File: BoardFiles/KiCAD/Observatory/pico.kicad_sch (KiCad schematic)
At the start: 2 parts, among them J31 Jumper, U5 Pico

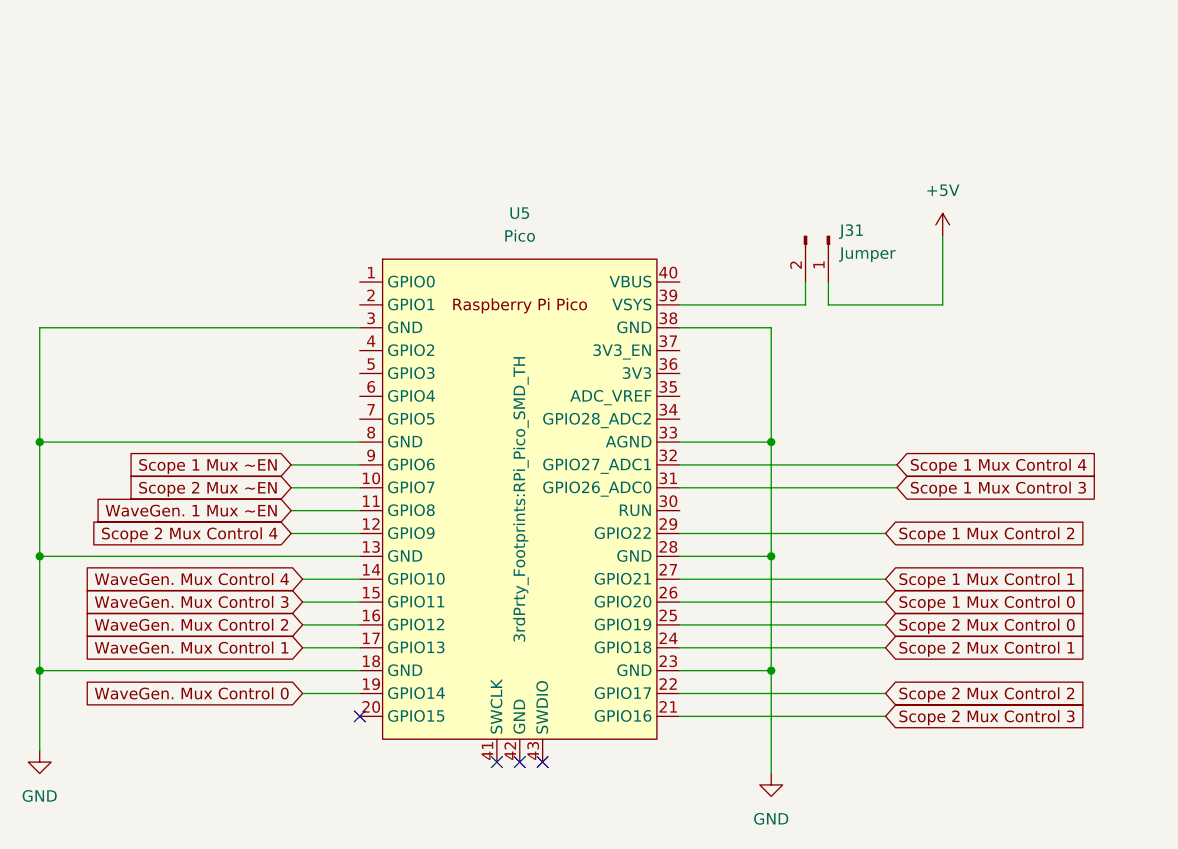
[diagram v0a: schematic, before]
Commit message: REV3 begin
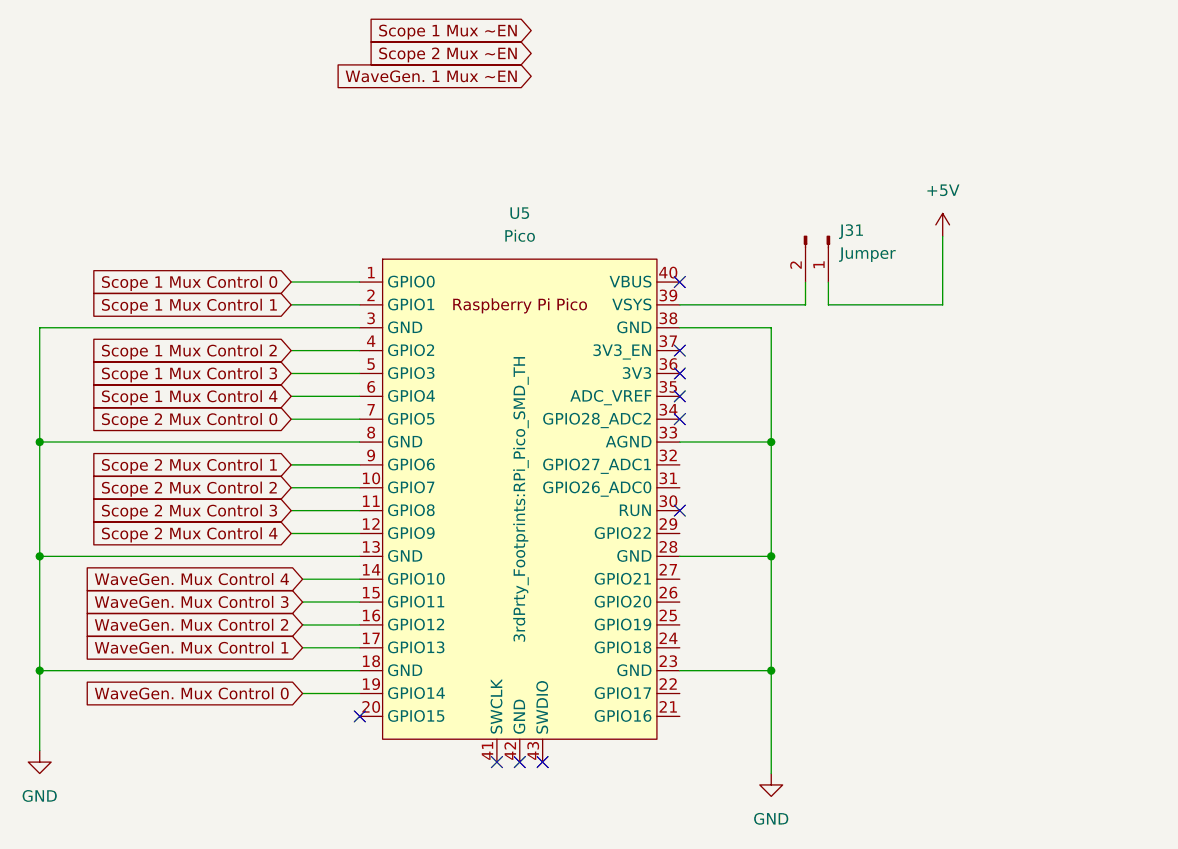
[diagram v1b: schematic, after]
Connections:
- net Scope 1 Mux Control 0: now also U5.1 (GPIO0); no longer U5.26 (GPIO20)
- net Scope 1 Mux Control 1: now also U5.2 (GPIO1); no longer U5.27 (GPIO21)
- net Scope 1 Mux Control 2: now also U5.4 (GPIO2); no longer U5.29 (GPIO22)
- net Scope 1 Mux Control 3: now also U5.5 (GPIO3); no longer U5.31 (GPIO26_ADC0)
- net Scope 1 Mux Control 4: now also U5.6 (GPIO4); no longer U5.32 (GPIO27_ADC1)
- net Scope 1 Mux ~EN: no longer U5.9 (GPIO6)
- net Scope 2 Mux Control 0: now also U5.7 (GPIO5); no longer U5.25 (GPIO19)
- net Scope 2 Mux Control 1: now also U5.9 (GPIO6); no longer U5.24 (GPIO18)
- net Scope 2 Mux Control 2: now also U5.10 (GPIO7); no longer U5.22 (GPIO17)
- net Scope 2 Mux Control 3: now also U5.11 (GPIO8); no longer U5.21 (GPIO16)
- net Scope 2 Mux ~EN: no longer U5.10 (GPIO7)
- net WaveGen. 1 Mux ~EN: no longer U5.11 (GPIO8)
- no-connect marks 4 -> 10

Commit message: REV3 DRC pass
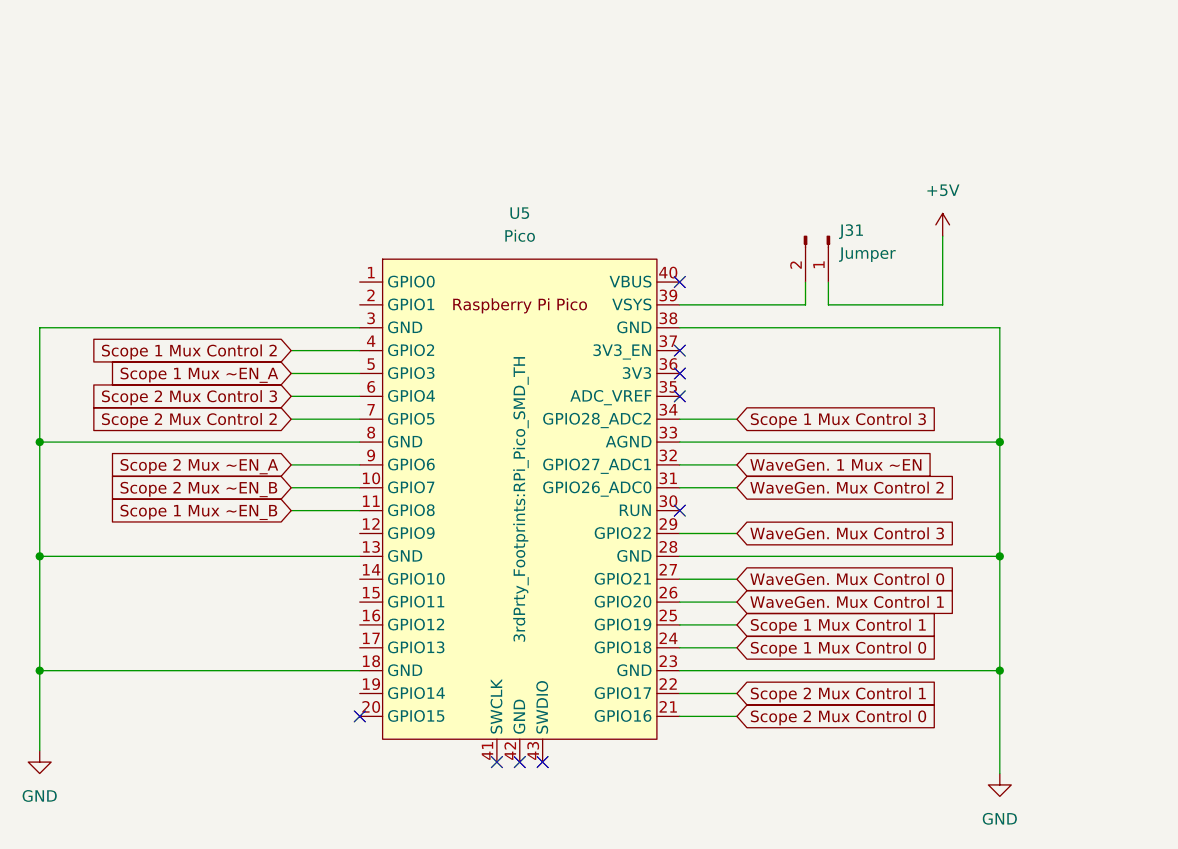
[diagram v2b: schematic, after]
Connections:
- net Scope 1 Mux Control 4 is gone; now on net Scope 2 Mux Control 3: U5.6 (GPIO4)
- net Scope 1 Mux Control 0: now also U5.24 (GPIO18); no longer U5.1 (GPIO0)
- net Scope 1 Mux Control 1: now also U5.25 (GPIO19); no longer U5.2 (GPIO1)
- net Scope 1 Mux Control 3: now also U5.34 (GPIO28_ADC2); no longer U5.5 (GPIO3)
- net Scope 2 Mux Control 0: now also U5.21 (GPIO16); no longer U5.7 (GPIO5)
- net Scope 2 Mux Control 1: now also U5.22 (GPIO17); no longer U5.9 (GPIO6)
- net Scope 2 Mux Control 2: now also U5.7 (GPIO5); no longer U5.10 (GPIO7)
- net Scope 2 Mux Control 3: no longer U5.11 (GPIO8)
- net WaveGen. 1 Mux ~EN: now also U5.32 (GPIO27_ADC1)
- net WaveGen. Mux Control 0: now also U5.27 (GPIO21); no longer U5.19 (GPIO14)
- net WaveGen. Mux Control 1: now also U5.26 (GPIO20); no longer U5.17 (GPIO13)
- net WaveGen. Mux Control 2: now also U5.31 (GPIO26_ADC0); no longer U5.16 (GPIO12)
- net WaveGen. Mux Control 3: now also U5.29 (GPIO22); no longer U5.15 (GPIO11)
- net Scope 2 Mux Control 4: no longer names the net of U5.12 (GPIO9)
- net WaveGen. Mux Control 4: no longer names the net of U5.14 (GPIO10)
- new net Scope 1 Mux ~EN_A: U5.5 (GPIO3)
- new net Scope 1 Mux ~EN_B: U5.11 (GPIO8)
- new net Scope 2 Mux ~EN_A: U5.9 (GPIO6)
- new net Scope 2 Mux ~EN_B: U5.10 (GPIO7)
- no-connect marks 10 -> 9
